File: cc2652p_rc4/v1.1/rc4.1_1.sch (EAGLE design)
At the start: 53 parts, among them IC3 CC2652R1FRGZ, Q1 SI2323DS, Q2 SI2323DS, Y1 Q22FA12800150, Y2 32.768KHz

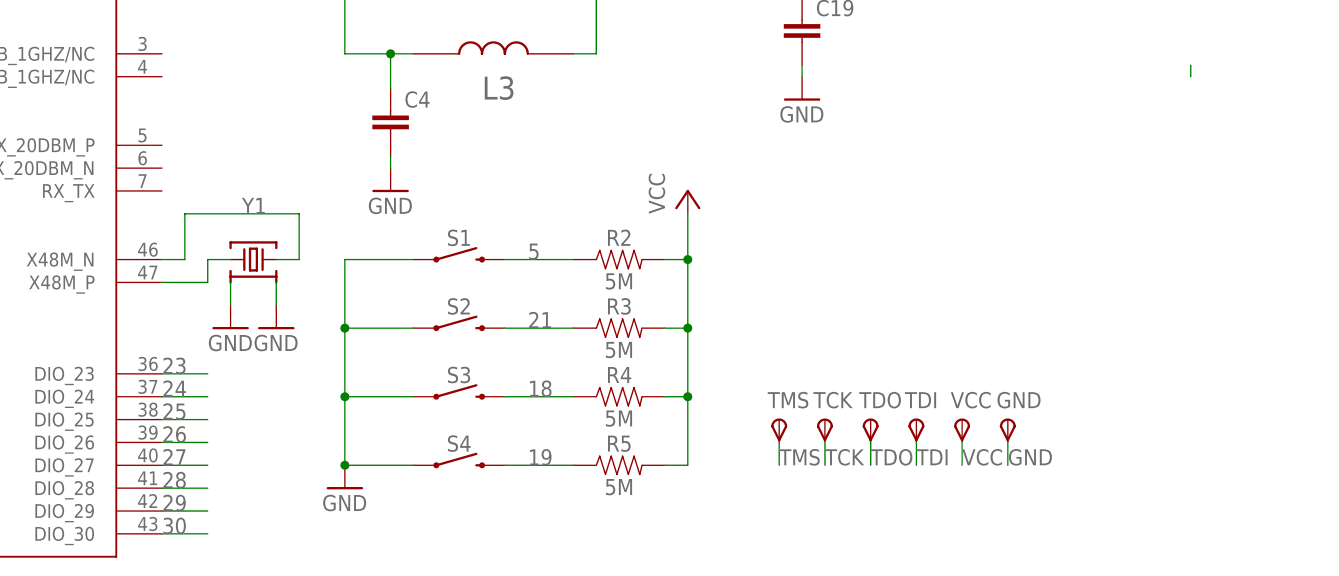
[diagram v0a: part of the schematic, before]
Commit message: Add files via upload
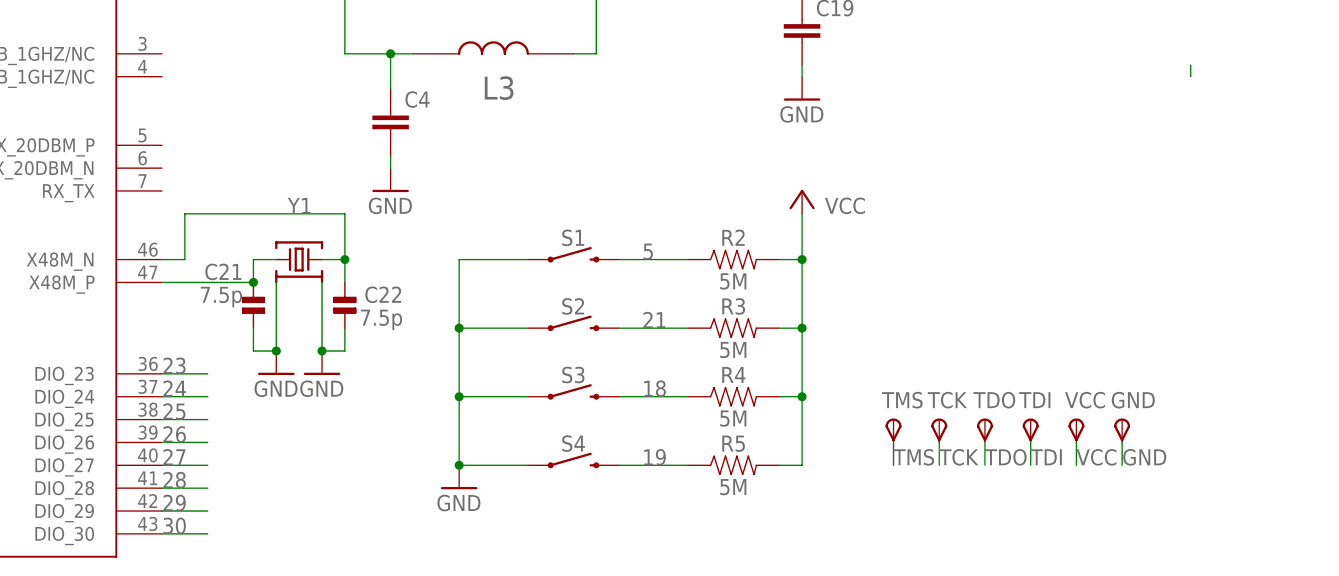
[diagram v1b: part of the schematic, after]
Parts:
- added C21, C22: 7.5p, ok-discretes-dev:CAP-0402
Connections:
- net GND: now also C21.1, C22.1
- net N$21: now also C21.2
- net N$4: now also C22.2
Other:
- moved on the sheet: GND, R2, R3, R4, R5, S1, S2, S3, S4, TCK, TDI, TDO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
